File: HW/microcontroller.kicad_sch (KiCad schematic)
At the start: 20 parts, among them J1 AVR-ISP-6, J7 Conn_01x04_Pin, U1 ATmega88P-20A, Y2 Crystal_GND24_Small

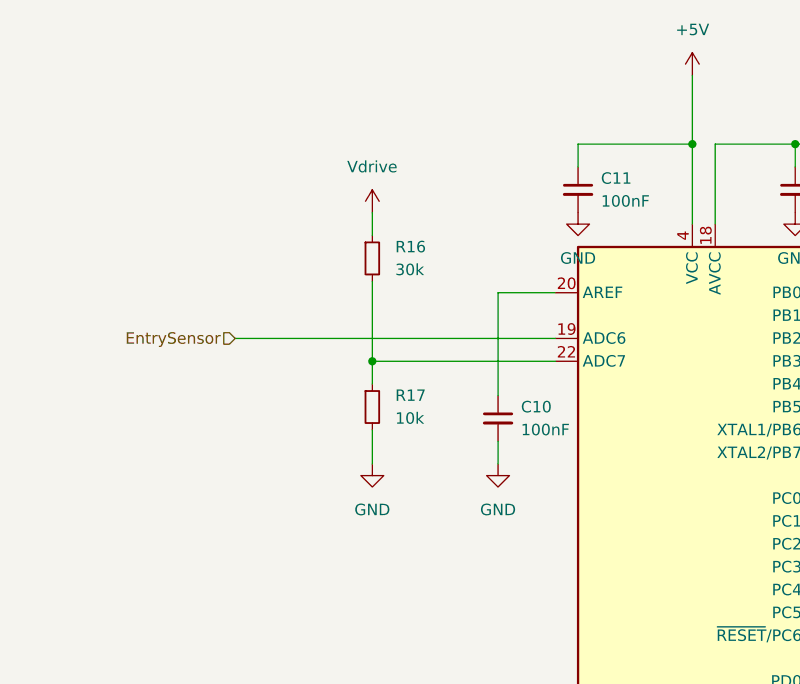
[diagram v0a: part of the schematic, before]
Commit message: update layout
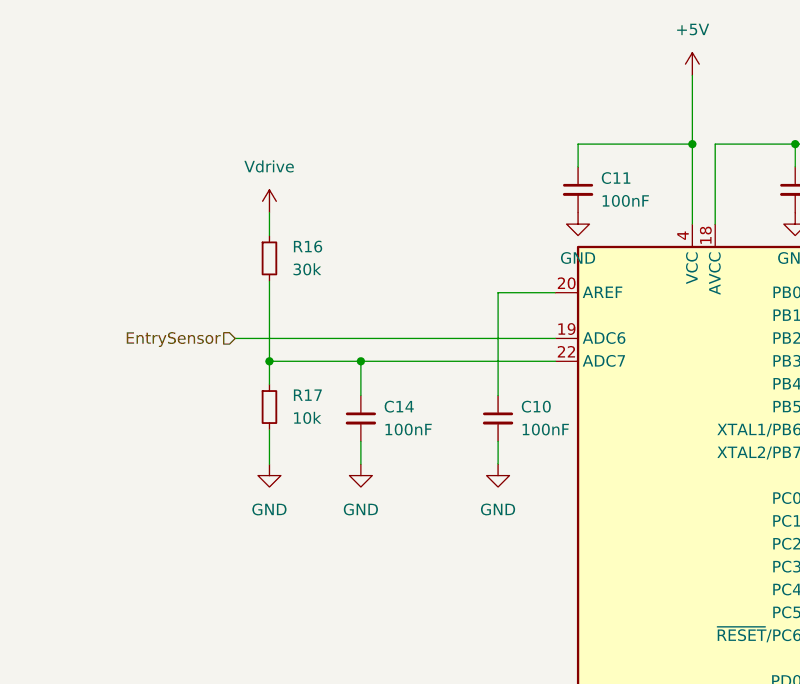
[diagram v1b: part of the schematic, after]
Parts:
- added C14: 100nF, Capacitor_SMD:C_0603_1608Metric_Pad1.08x0.95mm_HandSolder, symbol Device:C_Small
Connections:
- net GND: now also C14.2
- net at R16.2, R17.1, U1.22 (ADC7): now also C14.1
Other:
- moved on the sheet: R16, R17
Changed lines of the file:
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@@
 	)
 	(junction
+		(at 80.01 60.96)
+		(diameter 0)
+		(color 0 0 0 0)
+	)
+	(junction
 		(at 173.99 111.76)
 		(diameter 0)
@@
 	)
 	(junction
-		(at 81.28 60.96)
+		(at 69.85 60.96)
 		(diameter 0)
 		(color 0 0 0 0)
@@
 	(wire
 		(pts
+			(xy 80.01 69.85) (xy 80.01 72.39)
+		)
+		(stroke
+			(width 0)
+			(type default)
+		)
+	)
+	(wire
+		(pts
 			(xy 132.08 86.36) (xy 135.89 86.36)
 		)
@@
 	(wire
 		(pts
-			(xy 81.28 68.58) (xy 81.28 72.39)
+			(xy 69.85 68.58) (xy 69.85 72.39)
 		)
 		(stroke
@@
 	(wire
 		(pts
-			(xy 81.28 52.07) (xy 81.28 60.96)
+			(xy 69.85 52.07) (xy 69.85 60.96)
 		)
 		(stroke
@@
 	(wire
 		(pts
+			(xy 80.01 60.96) (xy 101.6 60.96)
+		)
+		(stroke
+			(width 0)
+			(type default)
+		)
+	)
+	(wire
+		(pts
 			(xy 128.27 36.83) (xy 137.16 36.83)
 		)
@@
 	(wire
 		(pts
-			(xy 81.28 44.45) (xy 81.28 46.99)
+			(xy 69.85 44.45) (xy 69.85 46.99)
 		)
 		(stroke
@@
 	(wire
 		(pts
+			(xy 80.01 60.96) (xy 80.01 64.77)
+		)
+		(stroke
+			(width 0)
+			(type default)
+		)
+	)
+	(wire
+		(pts
 			(xy 170.18 111.76) (xy 173.99 111.76)
 		)
@@
 	(wire
 		(pts
-			(xy 81.28 60.96) (xy 81.28 63.5)
+			(xy 69.85 60.96) (xy 69.85 63.5)
 		)
 		(stroke
@@
 	(wire
 		(pts
-			(xy 81.28 60.96) (xy 101.6 60.96)
+			(xy 69.85 60.96) (xy 80.01 60.96)
 		)
 		(stroke
@@
 	(symbol
 		(lib_id "Device:R_Small")
-		(at 81.28 66.04 0)
+		(at 69.85 66.04 0)
 		(unit 1)
 		(exclude_from_sim no)
@@
 		(fields_autoplaced yes)
 		(property "Reference" "R17"
-			(at 83.82 64.7699 0)
+			(at 72.39 64.7699 0)
 			(effects
 				(font
@@
 		)
 		(property "Value" "10k"
-			(at 83.82 67.3099 0)
+			(at 72.39 67.3099 0)
 			(effects
 				(font
@@
 		)
 		(property "Footprint" "Resistor_SMD:R_0603_1608Metric_Pad0.98x0.95mm_HandSolder"
-			(at 81.28 66.04 0)
+			(at 69.85 66.04 0)
 			(effects
 				(font
@@
 		)
 		(property "Datasheet" "~"
-			(at 81.28 66.04 0)
+			(at 69.85 66.04 0)
 			(effects
 				(font
@@
 		)
 		(property "Description" "Resistor, small symbol"
-			(at 81.28 66.04 0)
+			(at 69.85 66.04 0)
 			(effects
 				(font
@@
 	(symbol
 		(lib_id "power:Vdrive")
-		(at 81.28 44.45 0)
+		(at 69.85 44.45 0)
 		(unit 1)
 		(exclude_from_sim no)
@@
 		(fields_autoplaced yes)
 		(property "Reference" "#PWR050"
-			(at 81.28 48.26 0)
+			(at 69.85 48.26 0)
 			(effects
 				(font
@@
 		)
 		(property "Value" "Vdrive"
-			(at 81.28 39.37 0)
+			(at 69.85 39.37 0)
 			(effects
 				(font
@@
 		)
 		(property "Footprint" ""
-			(at 81.28 44.45 0)
+			(at 69.85 44.45 0)
 			(effects
 				(font
@@
 		)
 		(property "Datasheet" ""
-			(at 81.28 44.45 0)
+			(at 69.85 44.45 0)
 			(effects
 				(font
@@
 		)
 		(property "Description" "Power symbol creates a global label with name \"Vdrive\""
-			(at 81.28 44.45 0)
+			(at 69.85 44.45 0)
 			(effects
 				(font
@@
 	(symbol
 		(lib_id "power:GND")
-		(at 81.28 72.39 0)
+		(at 69.85 72.39 0)
 		(unit 1)
 		(exclude_from_sim no)
@@
 		(fields_autoplaced yes)
 		(property "Reference" "#PWR049"
-			(at 81.28 78.74 0)
+			(at 69.85 78.74 0)
 			(effects
 				(font
@@
 		)
 		(property "Value" "GND"
-			(at 81.28 77.47 0)
+			(at 69.85 77.47 0)
 			(effects
 				(font
@@
 		)
 		(property "Footprint" ""
-			(at 81.28 72.39 0)
+			(at 69.85 72.39 0)
 			(effects
 				(font
@@
 		)
 		(property "Datasheet" ""
-			(at 81.28 72.39 0)
+			(at 69.85 72.39 0)
 			(effects
 				(font
@@
 		)
 		(property "Description" "Power symbol creates a global label with name \"GND\" , ground"
-			(at 81.28 72.39 0)
+			(at 69.85 72.39 0)
 			(effects
 				(font
@@
 	)
 	(symbol
+		(lib_id "power:GND")
+		(at 80.01 72.39 0)
+		(unit 1)
+		(exclude_from_sim no)
+		(in_bom yes)
+		(on_board yes)
+		(dnp no)
+		(fields_autoplaced yes)
+		(property "Reference" "#PWR051"
+			(at 80.01 78.74 0)
+			(effects
+				(font
+					(size 1.27 1.27)
+				)
+				(hide yes)
+			)
+		)
+		(property "Value" "GND"
+			(at 80.01 77.47 0)
+			(effects
+				(font
+					(size 1.27 1.27)
+				)
+			)
+		)
+		(property "Footprint" ""
+			(at 80.01 72.39 0)
+			(effects
+				(font
+					(size 1.27 1.27)
+				)
+				(hide yes)
+			)
+		)
+		(property "Datasheet" ""
+			(at 80.01 72.39 0)
+			(effects
+				(font
+					(size 1.27 1.27)
+				)
+				(hide yes)
+			)
+		)
+		(property "Description" "Power symbol creates a global label with name \"GND\" , ground"
+			(at 80.01 72.39 0)
+			(effects
+				(font
+					(size 1.27 1.27)
+				)
+				(hide yes)
+			)
+		)
+		(pin "1"
+		)
+		(instances
+			(project "marble_accelerator"
+				(path "/338fb3bb-e550-4c92-aa76-5d93a75fae71/dfbdab4c-3176-4efa-832c-7a2279114595"
+					(reference "#PWR051")
+					(unit 1)
+				)
+			)
+		)
+	)
+	(symbol
 		(lib_id "Device:LED")
 		(at 154.94 111.76 180)
@@
 	(symbol
 		(lib_id "Device:C_Small")
+		(at 80.01 67.31 0)
+		(unit 1)
+		(exclude_from_sim no)
+		(in_bom yes)
+		(on_board yes)
+		(dnp no)
+		(fields_autoplaced yes)
+		(property "Reference" "C14"
+			(at 82.55 66.0462 0)
+			(effects
+				(font
+					(size 1.27 1.27)
+				)
+				(justify left)
+			)
+		)
+		(property "Value" "100nF"
+			(at 82.55 68.5862 0)
+			(effects
+				(font
+					(size 1.27 1.27)
+				)
+				(justify left)
+			)
+		)
+		(property "Footprint" "Capacitor_SMD:C_0603_1608Metric_Pad1.08x0.95mm_HandSolder"
+			(at 80.01 67.31 0)
+			(effects
+				(font
+					(size 1.27 1.27)
+				)
+				(hide yes)
+			)
+		)
+		(property "Datasheet" "~"
+			(at 80.01 67.31 0)
+			(effects
+				(font
+					(size 1.27 1.27)
+				)
+				(hide yes)
+			)
+		)
+		(property "Description" "Unpolarized capacitor, small symbol"
+			(at 80.01 67.31 0)
+			(effects
+				(font
+					(size 1.27 1.27)
+				)
+				(hide yes)
+			)
+		)
+		(pin "2"
+		)
+		(pin "1"
+		)
+		(instances
+			(project "marble_accelerator"
+				(path "/338fb3bb-e550-4c92-aa76-5d93a75fae71/dfbdab4c-3176-4efa-832c-7a2279114595"
+					(reference "C14")
+					(unit 1)
+				)
+			)
+		)
+	)
+	(symbol
+		(lib_id "Device:C_Small")
 		(at 95.25 67.31 0)
 		(unit 1)
@@
 	(symbol
 		(lib_id "Device:R_Small")
-		(at 81.28 49.53 0)
+		(at 69.85 49.53 0)
 		(unit 1)
 		(exclude_from_sim no)
@@
 		(fields_autoplaced yes)
 		(property "Reference" "R16"
-			(at 83.82 48.2599 0)
+			(at 72.39 48.2599 0)
 			(effects
 				(font
@@
 		)
 		(property "Value" "30k"
-			(at 83.82 50.7999 0)
+			(at 72.39 50.7999 0)
 			(effects
 				(font
@@
 		)
 		(property "Footprint" "Resistor_SMD:R_0603_1608Metric_Pad0.98x0.95mm_HandSolder"
-			(at 81.28 49.53 0)
+			(at 69.85 49.53 0)
 			(effects
 				(font
@@
 		)
 		(property "Datasheet" "~"
-			(at 81.28 49.53 0)
+			(at 69.85 49.53 0)
 			(effects
 				(font
@@
 		)
 		(property "Description" "Resistor, small symbol"
-			(at 81.28 49.53 0)
+			(at 69.85 49.53 0)
 			(effects
 				(font

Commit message: update layout and schematic
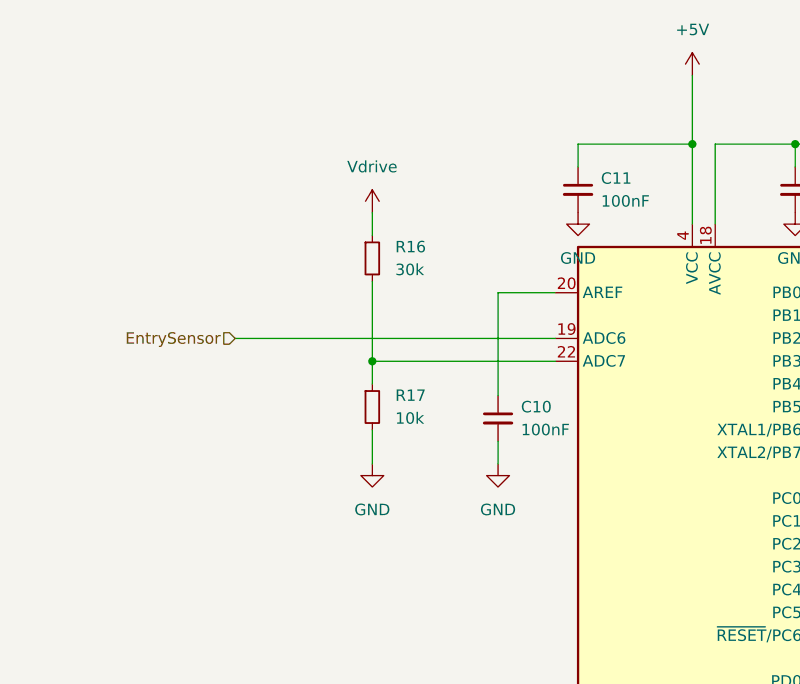
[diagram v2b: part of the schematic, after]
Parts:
- removed C14: 100nF, Capacitor_SMD:C_0603_1608Metric_Pad1.08x0.95mm_HandSolder, symbol Device:C_Small
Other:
- moved on the sheet: R16, R17
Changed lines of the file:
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@@
 	)
 	(junction
-		(at 80.01 60.96)
-		(diameter 0)
-		(color 0 0 0 0)
-	)
-	(junction
 		(at 173.99 111.76)
 		(diameter 0)
@@
 	)
 	(junction
-		(at 69.85 60.96)
+		(at 81.28 60.96)
 		(diameter 0)
 		(color 0 0 0 0)
@@
 	(wire
 		(pts
-			(xy 80.01 69.85) (xy 80.01 72.39)
-		)
-		(stroke
-			(width 0)
-			(type default)
-		)
-	)
-	(wire
-		(pts
 			(xy 132.08 86.36) (xy 135.89 86.36)
 		)
@@
 	(wire
 		(pts
-			(xy 69.85 68.58) (xy 69.85 72.39)
+			(xy 81.28 68.58) (xy 81.28 72.39)
 		)
 		(stroke
@@
 	(wire
 		(pts
-			(xy 69.85 52.07) (xy 69.85 60.96)
+			(xy 81.28 52.07) (xy 81.28 60.96)
 		)
 		(stroke
@@
 	(wire
 		(pts
-			(xy 80.01 60.96) (xy 101.6 60.96)
-		)
-		(stroke
-			(width 0)
-			(type default)
-		)
-	)
-	(wire
-		(pts
 			(xy 128.27 36.83) (xy 137.16 36.83)
 		)
@@
 	(wire
 		(pts
-			(xy 69.85 44.45) (xy 69.85 46.99)
+			(xy 81.28 44.45) (xy 81.28 46.99)
 		)
 		(stroke
@@
 	(wire
 		(pts
-			(xy 80.01 60.96) (xy 80.01 64.77)
-		)
-		(stroke
-			(width 0)
-			(type default)
-		)
-	)
-	(wire
-		(pts
 			(xy 170.18 111.76) (xy 173.99 111.76)
 		)
@@
 	(wire
 		(pts
-			(xy 69.85 60.96) (xy 69.85 63.5)
+			(xy 81.28 60.96) (xy 81.28 63.5)
 		)
 		(stroke
@@
 	(wire
 		(pts
-			(xy 69.85 60.96) (xy 80.01 60.96)
+			(xy 81.28 60.96) (xy 101.6 60.96)
 		)
 		(stroke
@@
 	(symbol
 		(lib_id "Device:R_Small")
-		(at 69.85 66.04 0)
+		(at 81.28 66.04 0)
 		(unit 1)
 		(exclude_from_sim no)
@@
 		(fields_autoplaced yes)
 		(property "Reference" "R17"
-			(at 72.39 64.7699 0)
+			(at 83.82 64.7699 0)
 			(effects
 				(font
@@
 		)
 		(property "Value" "10k"
-			(at 72.39 67.3099 0)
+			(at 83.82 67.3099 0)
 			(effects
 				(font
@@
 		)
 		(property "Footprint" "Resistor_SMD:R_0603_1608Metric_Pad0.98x0.95mm_HandSolder"
-			(at 69.85 66.04 0)
+			(at 81.28 66.04 0)
 			(effects
 				(font
@@
 		)
 		(property "Datasheet" "~"
-			(at 69.85 66.04 0)
+			(at 81.28 66.04 0)
 			(effects
 				(font
@@
 		)
 		(property "Description" "Resistor, small symbol"
-			(at 69.85 66.04 0)
+			(at 81.28 66.04 0)
 			(effects
 				(font
@@
 	(symbol
 		(lib_id "power:Vdrive")
-		(at 69.85 44.45 0)
+		(at 81.28 44.45 0)
 		(unit 1)
 		(exclude_from_sim no)
@@
 		(fields_autoplaced yes)
 		(property "Reference" "#PWR050"
-			(at 69.85 48.26 0)
+			(at 81.28 48.26 0)
 			(effects
 				(font
@@
 		)
 		(property "Value" "Vdrive"
-			(at 69.85 39.37 0)
+			(at 81.28 39.37 0)
 			(effects
 				(font
@@
 		)
 		(property "Footprint" ""
-			(at 69.85 44.45 0)
+			(at 81.28 44.45 0)
 			(effects
 				(font
@@
 		)
 		(property "Datasheet" ""
-			(at 69.85 44.45 0)
+			(at 81.28 44.45 0)
 			(effects
 				(font
@@
 		)
 		(property "Description" "Power symbol creates a global label with name \"Vdrive\""
-			(at 69.85 44.45 0)
+			(at 81.28 44.45 0)
 			(effects
 				(font
@@
 	(symbol
 		(lib_id "power:GND")
-		(at 69.85 72.39 0)
+		(at 81.28 72.39 0)
 		(unit 1)
 		(exclude_from_sim no)
@@
 		(fields_autoplaced yes)
 		(property "Reference" "#PWR049"
-			(at 69.85 78.74 0)
+			(at 81.28 78.74 0)
 			(effects
 				(font
@@
 		)
 		(property "Value" "GND"
-			(at 69.85 77.47 0)
+			(at 81.28 77.47 0)
 			(effects
 				(font
@@
 		)
 		(property "Footprint" ""
-			(at 69.85 72.39 0)
+			(at 81.28 72.39 0)
 			(effects
 				(font
@@
 		)
 		(property "Datasheet" ""
-			(at 69.85 72.39 0)
+			(at 81.28 72.39 0)
 			(effects
 				(font
@@
 		)
 		(property "Description" "Power symbol creates a global label with name \"GND\" , ground"
-			(at 69.85 72.39 0)
+			(at 81.28 72.39 0)
 			(effects
 				(font
@@
 	)
 	(symbol
-		(lib_id "power:GND")
-		(at 80.01 72.39 0)
-		(unit 1)
-		(exclude_from_sim no)
-		(in_bom yes)
-		(on_board yes)
-		(dnp no)
-		(fields_autoplaced yes)
-		(property "Reference" "#PWR051"
-			(at 80.01 78.74 0)
-			(effects
-				(font
-					(size 1.27 1.27)
-				)
-				(hide yes)
-			)
-		)
-		(property "Value" "GND"
-			(at 80.01 77.47 0)
-			(effects
-				(font
-					(size 1.27 1.27)
-				)
-			)
-		)
-		(property "Footprint" ""
-			(at 80.01 72.39 0)
-			(effects
-				(font
-					(size 1.27 1.27)
-				)
-				(hide yes)
-			)
-		)
-		(property "Datasheet" ""
-			(at 80.01 72.39 0)
-			(effects
-				(font
-					(size 1.27 1.27)
-				)
-				(hide yes)
-			)
-		)
-		(property "Description" "Power symbol creates a global label with name \"GND\" , ground"
-			(at 80.01 72.39 0)
-			(effects
-				(font
-					(size 1.27 1.27)
-				)
-				(hide yes)
-			)
-		)
-		(pin "1"
-		)
-		(instances
-			(project "marble_accelerator"
-				(path "/338fb3bb-e550-4c92-aa76-5d93a75fae71/dfbdab4c-3176-4efa-832c-7a2279114595"
-					(reference "#PWR051")
-					(unit 1)
-				)
-			)
-		)
-	)
-	(symbol
 		(lib_id "Device:LED")
 		(at 154.94 111.76 180)
@@
 	(symbol
 		(lib_id "Device:C_Small")
-		(at 80.01 67.31 0)
-		(unit 1)
-		(exclude_from_sim no)
-		(in_bom yes)
-		(on_board yes)
-		(dnp no)
-		(fields_autoplaced yes)
-		(property "Reference" "C14"
-			(at 82.55 66.0462 0)
-			(effects
-				(font
-					(size 1.27 1.27)
-				)
-				(justify left)
-			)
-		)
-		(property "Value" "100nF"
-			(at 82.55 68.5862 0)
-			(effects
-				(font
-					(size 1.27 1.27)
-				)
-				(justify left)
-			)
-		)
-		(property "Footprint" "Capacitor_SMD:C_0603_1608Metric_Pad1.08x0.95mm_HandSolder"
-			(at 80.01 67.31 0)
-			(effects
-				(font
-					(size 1.27 1.27)
-				)
-				(hide yes)
-			)
-		)
-		(property "Datasheet" "~"
-			(at 80.01 67.31 0)
-			(effects
-				(font
-					(size 1.27 1.27)
-				)
-				(hide yes)
-			)
-		)
-		(property "Description" "Unpolarized capacitor, small symbol"
-			(at 80.01 67.31 0)
-			(effects
-				(font
-					(size 1.27 1.27)
-				)
-				(hide yes)
-			)
-		)
-		(pin "2"
-		)
-		(pin "1"
-		)
-		(instances
-			(project "marble_accelerator"
-				(path "/338fb3bb-e550-4c92-aa76-5d93a75fae71/dfbdab4c-3176-4efa-832c-7a2279114595"
-					(reference "C14")
-					(unit 1)
-				)
-			)
-		)
-	)
-	(symbol
-		(lib_id "Device:C_Small")
 		(at 95.25 67.31 0)
 		(unit 1)
@@
 	(symbol
 		(lib_id "Device:R_Small")
-		(at 69.85 49.53 0)
+		(at 81.28 49.53 0)
 		(unit 1)
 		(exclude_from_sim no)
@@
 		(fields_autoplaced yes)
 		(property "Reference" "R16"
-			(at 72.39 48.2599 0)
+			(at 83.82 48.2599 0)
 			(effects
 				(font
@@
 		)
 		(property "Value" "30k"
-			(at 72.39 50.7999 0)
+			(at 83.82 50.7999 0)
 			(effects
 				(font
@@
 		)
 		(property "Footprint" "Resistor_SMD:R_0603_1608Metric_Pad0.98x0.95mm_HandSolder"
-			(at 69.85 49.53 0)
+			(at 81.28 49.53 0)
 			(effects
 				(font
@@
 		)
 		(property "Datasheet" "~"
-			(at 69.85 49.53 0)
+			(at 81.28 49.53 0)
 			(effects
 				(font
@@
 		)
 		(property "Description" "Resistor, small symbol"
-			(at 69.85 49.53 0)
+			(at 81.28 49.53 0)
 			(effects
 				(font
